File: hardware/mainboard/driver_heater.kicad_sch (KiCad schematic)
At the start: 8 parts, among them J18 Screw_Terminal_01x02, Q1 AGM308MBP, SW9 SW_SPDT

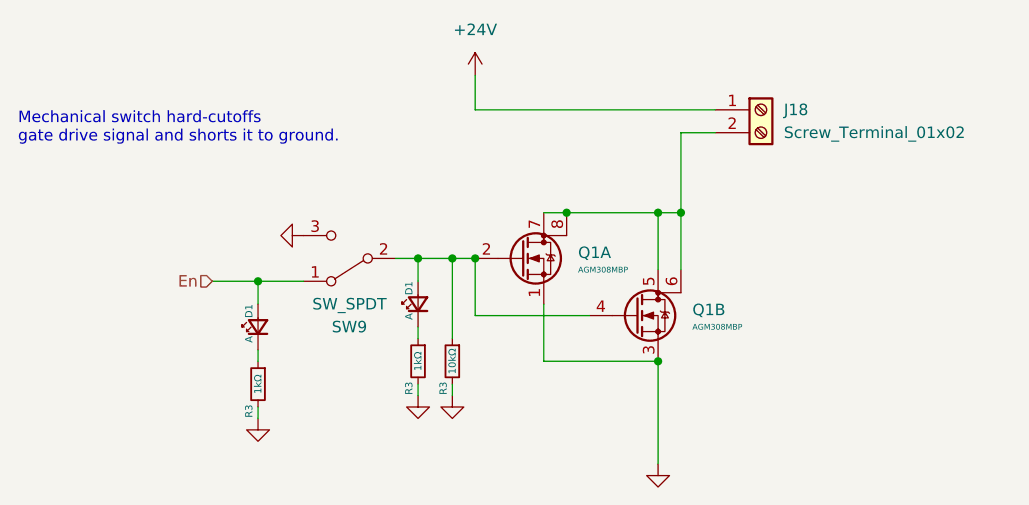
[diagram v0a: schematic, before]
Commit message: redoing board for version alpha 0.2
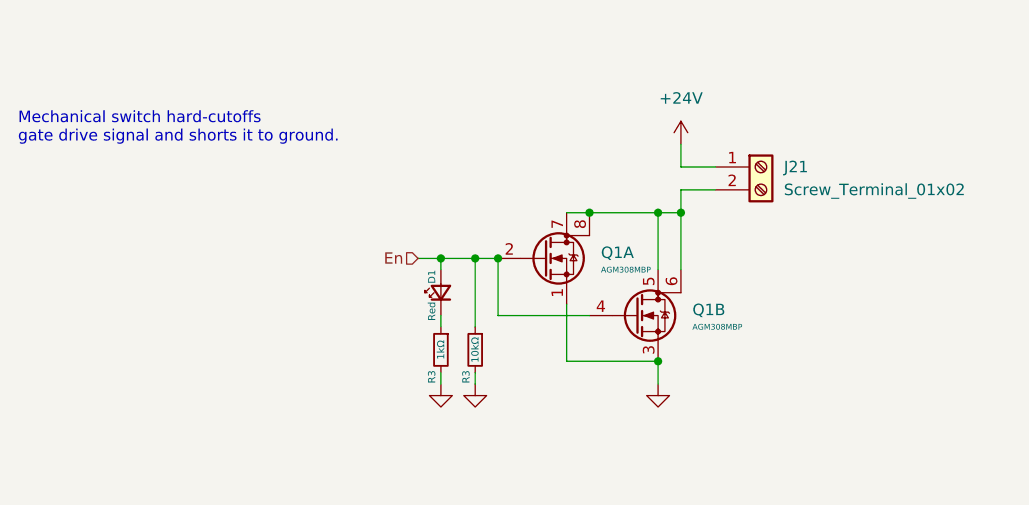
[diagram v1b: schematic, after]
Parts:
- removed D1 (x2): A, AlphaLib:0603LED, symbol Device:LED_Small
- removed R3 (x2): 1kΩ, AlphaLib:0402R, symbol Device:R_Small
- removed R3: 10kΩ, AlphaLib:0402R, symbol Device:R_Small
- removed SW9: SW_SPDT, corevus:MSS12C02-LS, symbol Switch:SW_SPDT
- added D1: Red, AlphaLib:0402LED, symbol Device:LED_Small
- added R3: 10kΩ, AlphaLib:0402R, symbol Device:R_Small
- added R3: 1kΩ, AlphaLib:0402R, symbol Device:R_Small
- renumbered J18 to J21
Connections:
- net En: now also Q1.2 (G), Q1.4 (G), D1.2 (A), R3.1
- net GND: now also R3.2, R3.2
- new net: D1.1 (K), R3.1
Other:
- moved on the sheet: J21, Q1A
